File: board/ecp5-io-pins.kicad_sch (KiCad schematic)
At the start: 9 parts

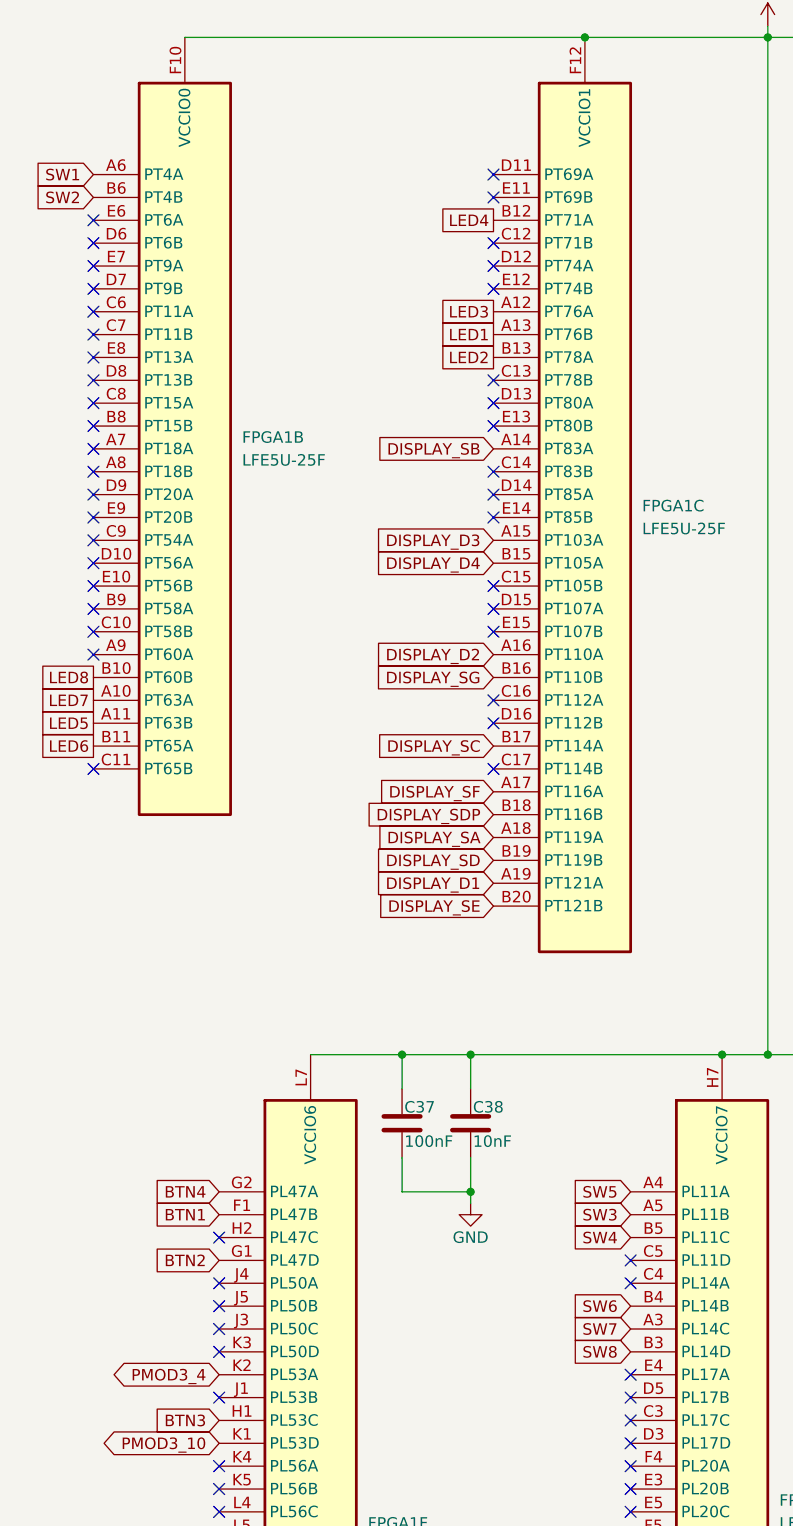
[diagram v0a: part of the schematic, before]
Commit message: Change switches
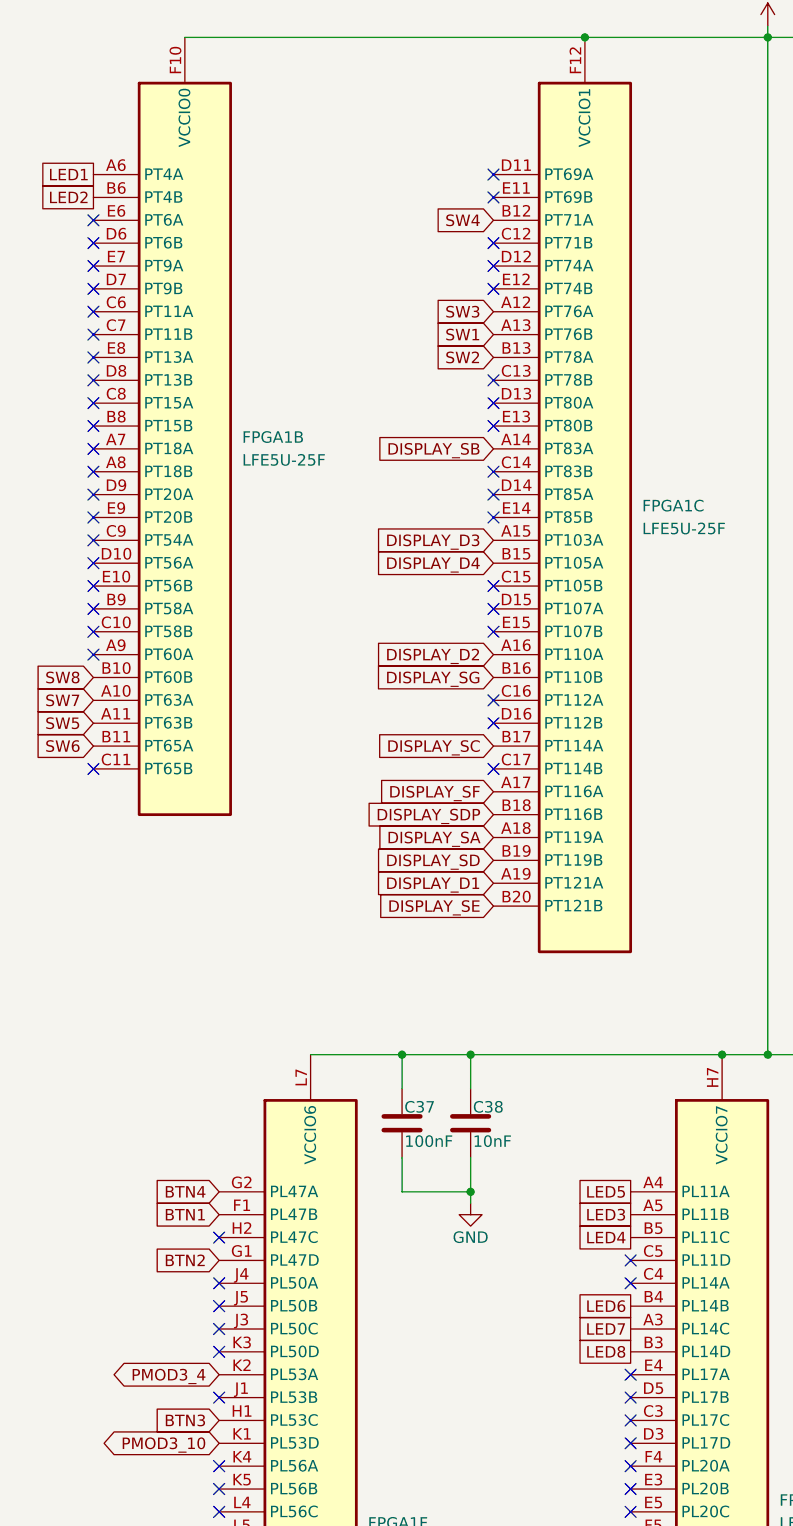
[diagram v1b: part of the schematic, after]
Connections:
- net LED1: now also FPGA1.A6 (PT4A); no longer FPGA1.A13 (PT76B)
- net LED2: now also FPGA1.B6 (PT4B); no longer FPGA1.B13 (PT78A)
- net LED3: now also FPGA1.A5 (PL11B); no longer FPGA1.A12 (PT76A)
- net LED4: now also FPGA1.B5 (PL11C); no longer FPGA1.B12 (PT71A)
- net LED5: now also FPGA1.A4 (PL11A); no longer FPGA1.A11 (PT63B)
- net LED6: now also FPGA1.B4 (PL14B); no longer FPGA1.B11 (PT65A)
- net LED7: now also FPGA1.A3 (PL14C); no longer FPGA1.A10 (PT63A)
- net LED8: now also FPGA1.B3 (PL14D); no longer FPGA1.B10 (PT60B)
- net SW1: now also FPGA1.A13 (PT76B); no longer FPGA1.A6 (PT4A)
- net SW2: now also FPGA1.B13 (PT78A); no longer FPGA1.B6 (PT4B)
- net SW3: now also FPGA1.A12 (PT76A); no longer FPGA1.A5 (PL11B)
- net SW4: now also FPGA1.B12 (PT71A); no longer FPGA1.B5 (PL11C)
- net SW5: now also FPGA1.A11 (PT63B); no longer FPGA1.A4 (PL11A)
- net SW6: now also FPGA1.B11 (PT65A); no longer FPGA1.B4 (PL14B)
- net SW7: now also FPGA1.A10 (PT63A); no longer FPGA1.A3 (PL14C)
- net SW8: now also FPGA1.B10 (PT60B); no longer FPGA1.B3 (PL14D)
